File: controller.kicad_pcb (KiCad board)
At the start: 2 copper layers, 29 parts, among them J1 Conn_ST_STDC14, J2 USB_C_Receptacle_USB2.0_14P, SW1 SW_Push, SW2 SW_Push, U1 STM32L476RGTx, U2 BD33FC0FP, U3 NUP2202

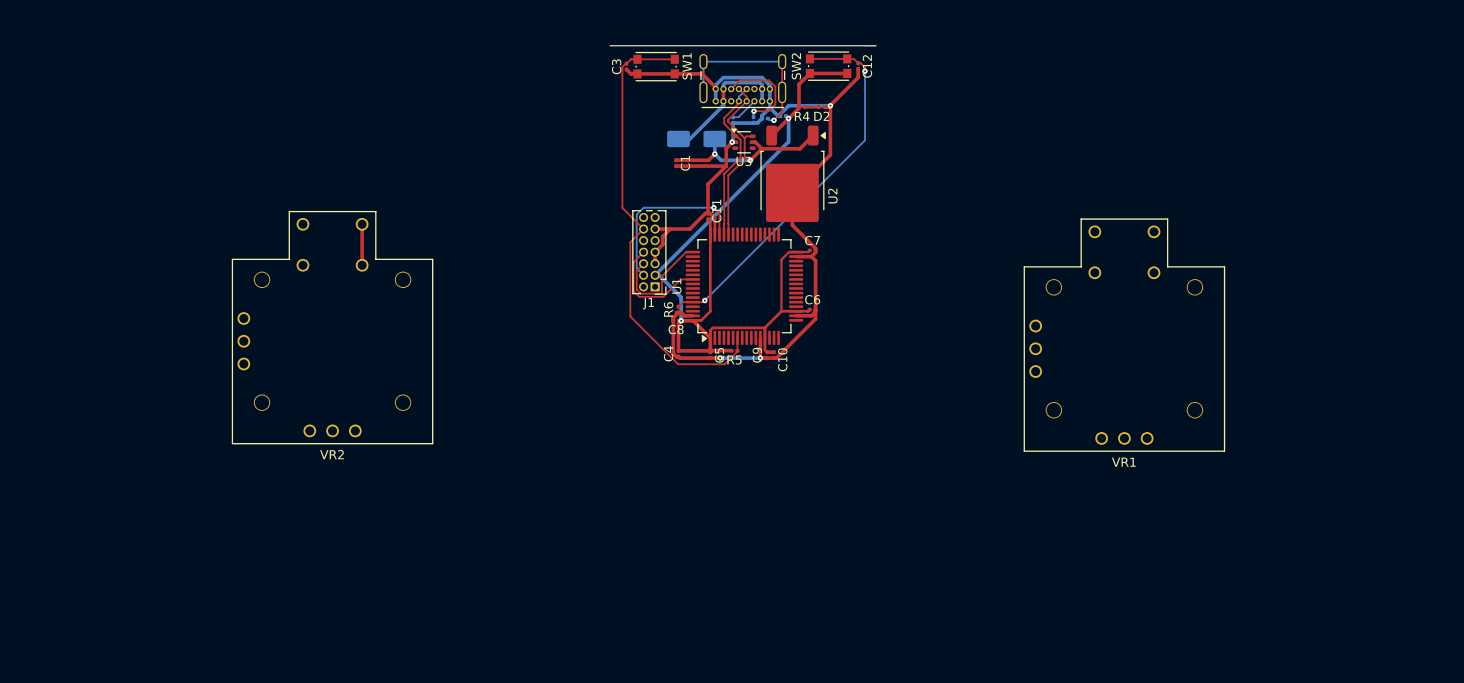
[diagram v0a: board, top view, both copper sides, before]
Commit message: finish routing, more or less
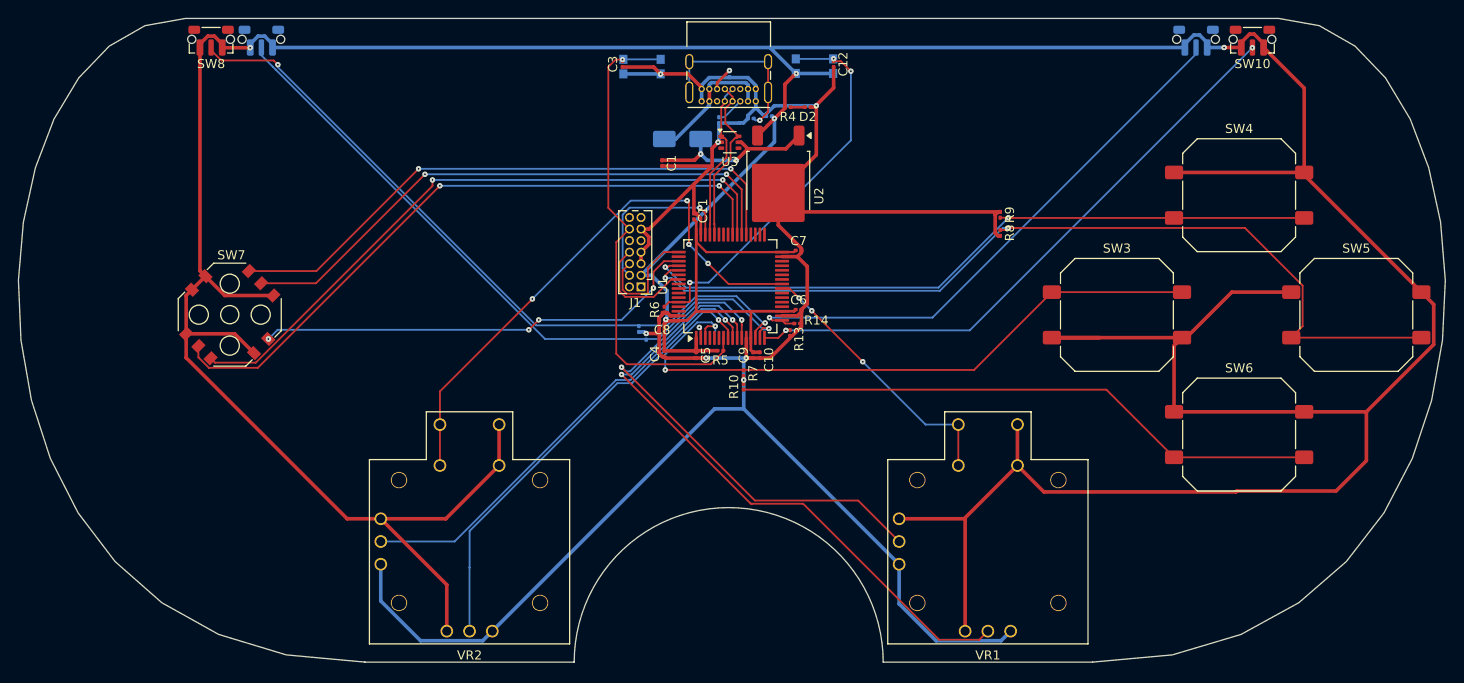
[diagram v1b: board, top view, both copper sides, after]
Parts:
- added R10: 10k, Resistor_SMD:R_0201_0603Metric, F.Cu at (138.9, 102.6)
- added R11: 10k, Resistor_SMD:R_0201_0603Metric, B.Cu at (127.4, 96.3)
- added R12: 10k, Resistor_SMD:R_0201_0603Metric, B.Cu at (128.2, 97.2)
- added R13: 10k, Resistor_SMD:R_0201_0603Metric, F.Cu at (144.0, 96.7)
- added R14: 10k, Resistor_SMD:R_0201_0603Metric, F.Cu at (144.8, 95.7)
- added R7: 10k, Resistor_SMD:R_0201_0603Metric, F.Cu at (138.9, 101.2)
- added R8: 10k, Resistor_SMD:R_0201_0603Metric, F.Cu at (167.1, 85.7)
- added R9: 10k, Resistor_SMD:R_0201_0603Metric, F.Cu at (167.1, 83.8)
- added SW10: SW_Push, Button_Switch_SMD:SW_Push_1P1T-MP_NO_Horizontal_Alps_SKRTLAE010, F.Cu at (194.8, 64.5)
- added SW11: SW_Push, Button_Switch_SMD:SW_Push_1P1T-MP_NO_Horizontal_Alps_SKRTLAE010, B.Cu at (188.6, 64.5)
- added SW3: SW_Push, Button_Switch_SMD:SW_Push_1P1T_NO_CK_PTS125Sx43SMTR, F.Cu at (179.9, 94.8)
- added SW4: SW_Push, Button_Switch_SMD:SW_Push_1P1T_NO_CK_PTS125Sx43SMTR, F.Cu at (193.3, 81.6)
- added SW5: SW_Push, Button_Switch_SMD:SW_Push_1P1T_NO_CK_PTS125Sx43SMTR, F.Cu at (206.2, 94.8)
- added SW6: SW_Push, Button_Switch_SMD:SW_Push_1P1T_NO_CK_PTS125Sx43SMTR, F.Cu at (193.3, 107.9)
- added SW7: ~, K1-1210UN-01:K1-1210UN-01, F.Cu at (82.5, 94.7)
- added SW8: SW_Push, Button_Switch_SMD:SW_Push_1P1T-MP_NO_Horizontal_Alps_SKRTLAE010, F.Cu at (80.4, 64.5)
- added SW9: SW_Push, Button_Switch_SMD:SW_Push_1P1T-MP_NO_Horizontal_Alps_SKRTLAE010, B.Cu at (85.9, 64.5)
- SW1, SW2: moved to B.Cu
- moved VR2 26.7 mm to (108.8, 119.6)
- moved VR1 26.0 mm to (165.7, 119.6)
- moved R2 5.68 mm to (137.3, 68.3)
- moved C12 2.71 mm to (148.8, 67.2)
- moved C1 1.55 mm to (129.9, 78.1)
- moved C10 1.55 mm to (140.7, 99.2)
- moved C11 1.55 mm to (133.4, 83.9)
- moved C2 1.55 mm to (141.7, 72.9)
- moved C4 1.55 mm to (130.2, 99.0)
- moved C5 1.55 mm to (133.7, 99.2)
- moved C6 1.55 mm to (144.9, 94.2)
- moved C7 1.55 mm to (144.9, 87.7)
- moved C8 1.55 mm to (130.0, 95.4)
- moved C9 1.55 mm to (139.9, 99.2)
- moved D1 1.55 mm to (132.2, 75.4)
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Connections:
- U1 pad 10: LeftX -> RightX
- U1 pad 11: LeftY -> RightY
- U1 pad 14: unconnected-(U1-PA0-Pad14) -> LeftTriggerTop
- U1 pad 15: unconnected-(U1-PA1-Pad15) -> LeftTriggerBottom
- U1 pad 16: unconnected-(U1-PA2-Pad16) -> RightTriggerTop
- U1 pad 17: unconnected-(U1-PA3-Pad17) -> RightTriggerBottom
- U1 pad 2: unconnected-(U1-PC13-Pad2) -> ButtonDown
- U1 pad 20: unconnected-(U1-PA4-Pad20) -> SelectINS
- U1 pad 21: unconnected-(U1-PA5-Pad21) -> SPI1_SCK
- U1 pad 22: unconnected-(U1-PA6-Pad22) -> SPI1_MISO
- U1 pad 23: unconnected-(U1-PA7-Pad23) -> SPI1_MOSI
- U1 pad 3: unconnected-(U1-PC14-Pad3) -> ButtonLeft
- U1 pad 37: unconnected-(U1-PC6-Pad37) -> DPadUp
- U1 pad 38: unconnected-(U1-PC7-Pad38) -> DPadRight
- U1 pad 39: unconnected-(U1-PC8-Pad39) -> DPadDown
- U1 pad 40: unconnected-(U1-PC9-Pad40) -> DPadLeft
- U1 pad 51: unconnected-(U1-PC10-Pad51) -> DPadCenter
- U1 pad 52: unconnected-(U1-PC11-Pad52) -> ButtonUp
- U1 pad 53: unconnected-(U1-PC12-Pad53) -> ButtonRight
- U1 pad 8: RightX -> LeftX
- U1 pad 9: RightY -> LeftY
- VR1 pad 3: Net-(VR1-VSS) -> GND
- VR1 pad 3': Net-(VR1-VSS') -> GND
- VR2 pad 3: Net-(VR2-VSS) -> GND
- VR2 pad 3': Net-(VR2-VSS') -> GND
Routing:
- net +3.3V: track 101.2 -> 547.4 mm, vias 2 -> 5
- net GND: track 128.4 -> 269.3 mm, vias 4 -> 7
- net ButtonRight: track 0.00 -> 99.6 mm, vias 0 -> 2
- net LeftTriggerTop: track 0.00 -> 78.7 mm, vias 0 -> 2
- net ButtonUp: track 0.00 -> 76.9 mm, vias 0 -> 2
- net LeftTriggerBottom: track 0.00 -> 74.7 mm, vias 0 -> 1
- net DPadLeft: track 0.00 -> 73.2 mm, vias 0 -> 2
- net ButtonLeft: track 0.00 -> 71.9 mm, vias 0 -> 2
- net DPadDown: track 0.00 -> 71.9 mm, vias 0 -> 2
- net RightX: track 0.00 -> 70.9 mm, vias 0 -> 2
- net RightTriggerTop: track 0.00 -> 67.3 mm, vias 0 -> 2
- net ButtonDown: track 0.00 -> 66.0 mm, vias 0 -> 1
- net DPadUp: track 0.00 -> 65.5 mm, vias 0 -> 2
- net DPadRight: track 0.00 -> 63.4 mm, vias 0 -> 2
- net RightTriggerBottom: track 0.00 -> 62.6 mm, vias 0 -> 1
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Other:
- board outline added: 156.8 x 70.7 mm
- board text added: "RESET"
